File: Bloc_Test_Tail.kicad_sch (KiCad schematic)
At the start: 44 parts, among them Q10 2N7000, Q5 2N7000, Q6 2N7000, Q7 2N7000, Q8 2N7000, Q9 2N7000

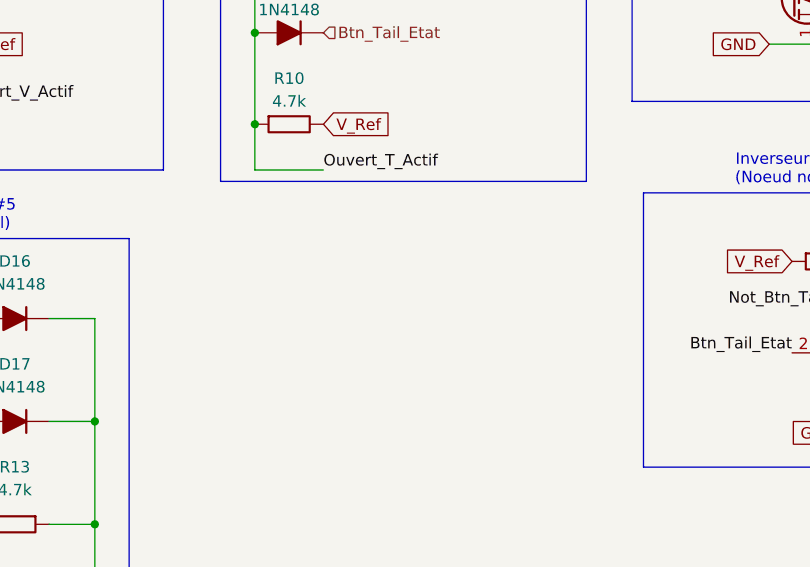
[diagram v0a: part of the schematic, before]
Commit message: Add files via upload
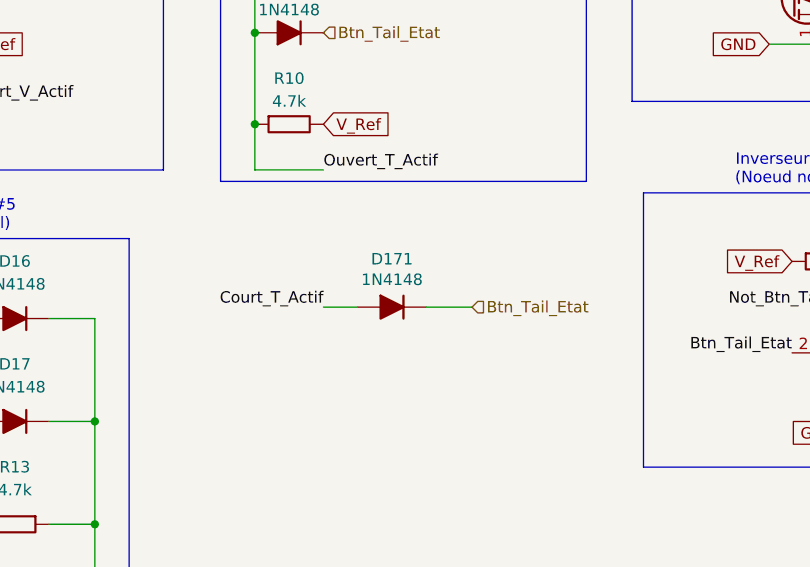
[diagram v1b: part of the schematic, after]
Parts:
- added D171: 1N4148, PCM_Diode_THT_AKL:D_DO-35_SOD27_P7.62mm_Horizontal, symbol PCM_Diode_AKL:1N4148
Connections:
- net Btn_Tail_Etat: now also D171.1 (K)
- net Court_T_Actif: now also D171.2 (A)
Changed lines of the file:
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@@
 	(wire
 		(pts
+			(xy 118.11 115.57) (xy 123.19 115.57)
+		)
+		(stroke
+			(width 0)
+			(type default)
+		)
+	)
+	(wire
+		(pts
 			(xy 81.28 116.84) (xy 76.2 116.84)
 		)
@@
 	(wire
 		(pts
+			(xy 106.68 115.57) (xy 110.49 115.57)
+		)
+		(stroke
+			(width 0)
+			(type default)
+		)
+	)
+	(wire
+		(pts
 			(xy 114.3 191.77) (xy 121.92 191.77)
 		)
@@
 		)
 	)
+	(label "Court_T_Actif"
+		(at 106.68 115.57 180)
+		(effects
+			(font
+				(size 1.27 1.27)
+			)
+			(justify right bottom)
+		)
+	)
 	(label "Fault_Actif"
 		(at 220.98 125.73 0)
@@
 		)
 	)
+	(hierarchical_label "Btn_Tail_Etat"
+		(shape input)
+		(at 123.19 115.57 0)
+		(effects
+			(font
+				(size 1.27 1.27)
+			)
+			(justify left)
+		)
+	)
 	(hierarchical_label "Court_Tail_Vehic"
 		(shape input)
@@
 					(unit 1)
 				)
+			)
+		)
+	)
+	(symbol
+		(lib_id "PCM_Diode_AKL:1N4148")
+		(at 114.3 115.57 0)
+		(unit 1)
+		(body_style 1)
+		(exclude_from_sim no)
+		(in_bom yes)
+		(on_board yes)
+		(in_pos_files yes)
+		(dnp no)
+		(property "Reference" "D171"
+			(at 114.3 110.236 0)
+			(show_name no)
+			(do_not_autoplace no)
+			(effects
+				(font
+					(size 1.27 1.27)
+				)
+			)
+		)
+		(property "Value" "1N4148"
+			(at 114.3 112.522 0)
+			(show_name no)
+			(do_not_autoplace no)
+			(effects
+				(font
+					(size 1.27 1.27)
+				)
+			)
+		)
+		(property "Footprint" "PCM_Diode_THT_AKL:D_DO-35_SOD27_P7.62mm_Horizontal"
+			(at 114.3 115.57 0)
+			(hide yes)
+			(show_name no)
+			(do_not_autoplace no)
+			(effects
+				(font
+					(size 1.27 1.27)
+				)
+			)
+		)
+		(property "Datasheet" "https://datasheet.octopart.com/1N4148TR-ON-Semiconductor-datasheet-42765246.pdf"
+			(at 114.3 115.57 0)
+			(hide yes)
+			(show_name no)
+			(do_not_autoplace no)
+			(effects
+				(font
+					(size 1.27 1.27)
+				)
+			)
+		)
+		(property "Description" "DO-35 Diode, Small Signal, Fast Switching, 75V, 150mA, 4ns, Alternate KiCad Library"
+			(at 114.3 115.57 0)
+			(hide yes)
+			(show_name no)
+			(do_not_autoplace no)
+			(effects
+				(font
+					(size 1.27 1.27)
+				)
+			)
+		)
+		(pin "2"
+		)
+		(pin "1"
+		)
+		(instances
+			(project "TrailerDiagnosticSystem"
+				(path "/d4e407a7-3e32-4226-ae57-831ecdb3edf4/891824ea-a79b-4938-b55f-b811c31e662c/16a46d25-c71f-43e3-999b-a92ed112d481"
+					(reference "D171")
+					(unit 1)
+				)
